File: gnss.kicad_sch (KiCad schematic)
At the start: 73 parts, among them J7 Conn_Coaxial, J8 Conn_Coaxial_Small, Q8 AO3401A, Q9 BSS138, SW4 SW_Push, SW5 SW_Push, U10 TPS259474LRPWR, U8 NEO-M9N, U9 TPS7A2033PDBVR

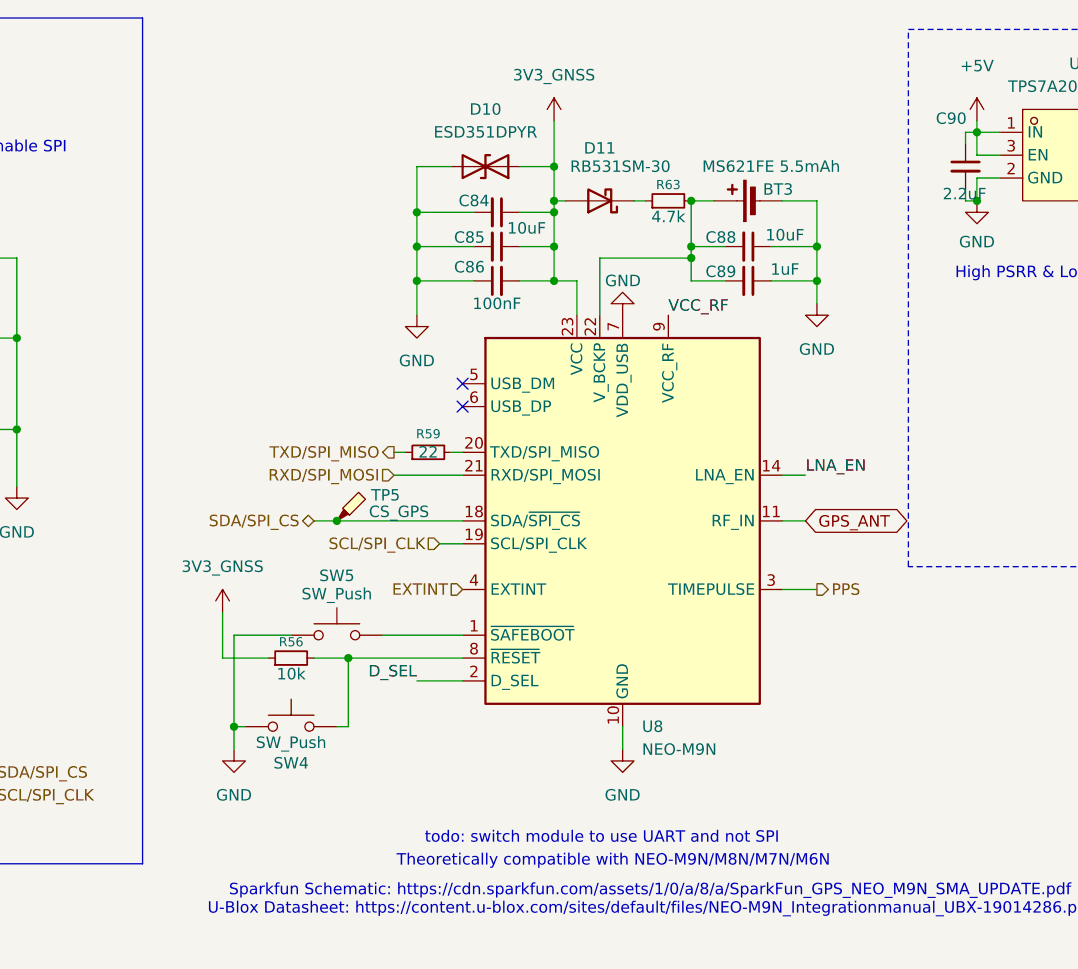
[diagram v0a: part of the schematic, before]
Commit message: e-ink
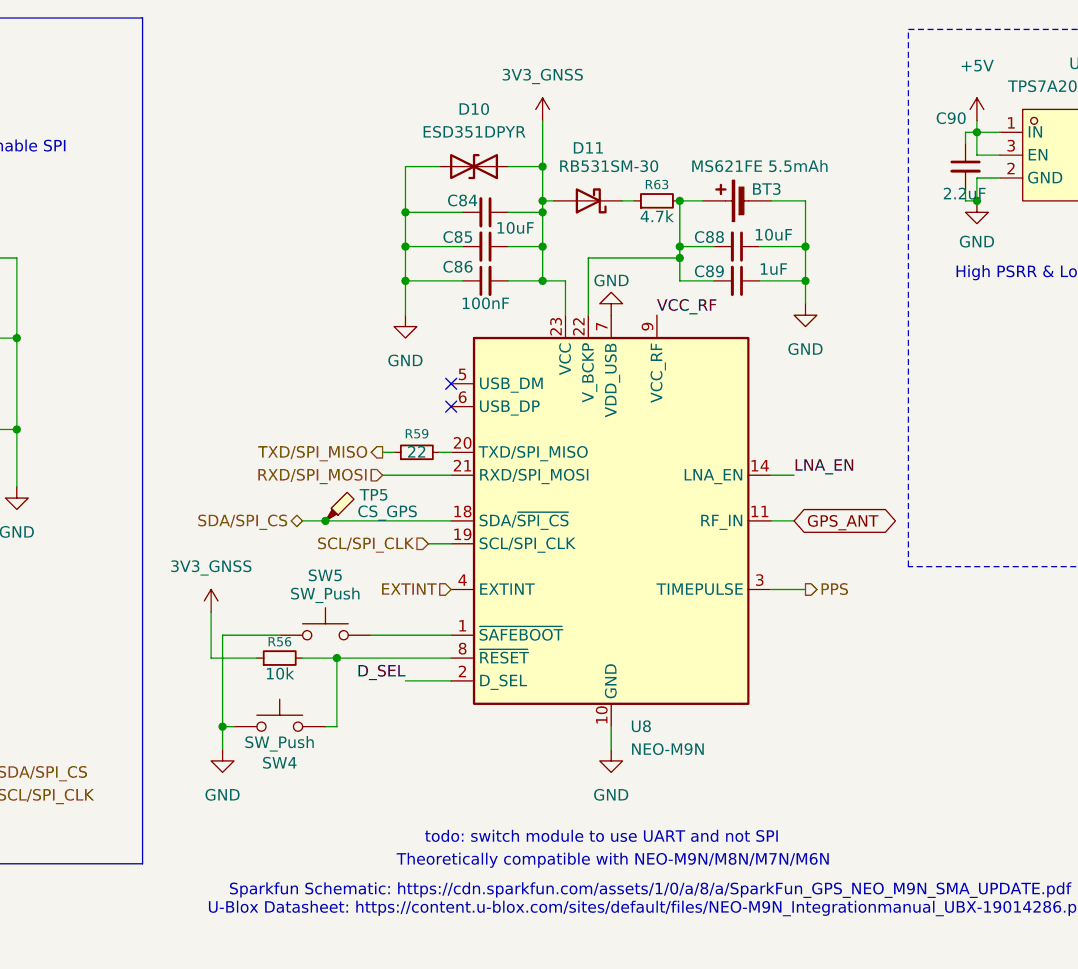
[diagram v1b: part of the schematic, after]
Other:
- moved on the sheet: BT3, C84, C85, C86, C88, C89, D10, D11, R56, R59, R63, SW4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
